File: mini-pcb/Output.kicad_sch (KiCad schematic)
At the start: 13 parts, among them U2 OPA1664D

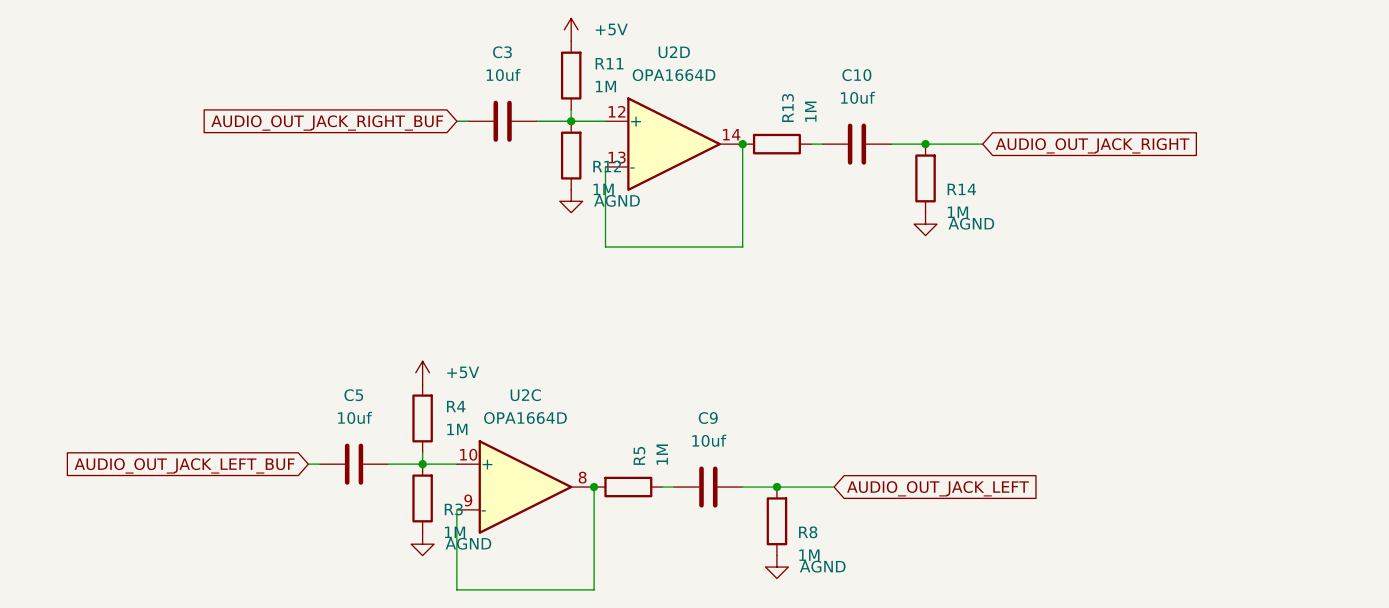
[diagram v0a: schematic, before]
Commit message: almost done with mini pcb
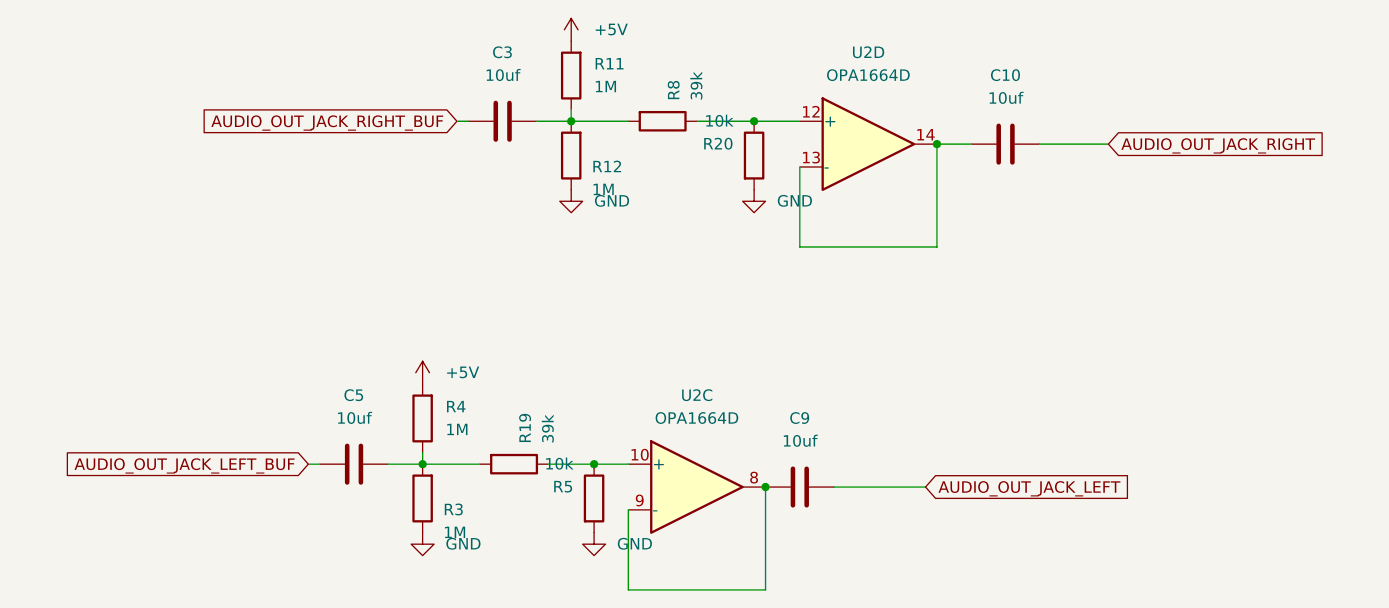
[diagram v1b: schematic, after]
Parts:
- removed R13, R14: 1M, Resistor_SMD:R_0603_1608Metric, symbol Device:R
- added R19: 39k, Resistor_SMD:R_0603_1608Metric, symbol Device:R
- added R20: 10k, Resistor_SMD:R_0603_1608Metric, symbol Device:R
- R5: value 1M -> 10k
- R8: value 1M -> 39k
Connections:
- net AUDIO_OUT_JACK_LEFT: no longer R8.2
- net at C9.1: now also U2.8, U2.9 (-); no longer R5.1
- net at C5.2, R3.2, R4.1: now also R19.2; no longer U2.10 (+)
- net at C3.2, R11.1, R12.2: now also R8.2; no longer U2.12 (+)
- net at C10.1: now also U2.13 (-), U2.14
- net AGND renamed GND
- net GND: now also R5.2, R20.2; no longer R8.1
- new net: R19.1, R5.1, U2.10 (+)
- new net: R20.1, R8.1, U2.12 (+)
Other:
- moved on the sheet: C10, C9, U2C, U2D
